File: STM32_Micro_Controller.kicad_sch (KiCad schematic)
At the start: 1 part, among them U1 STM32F103C8T6

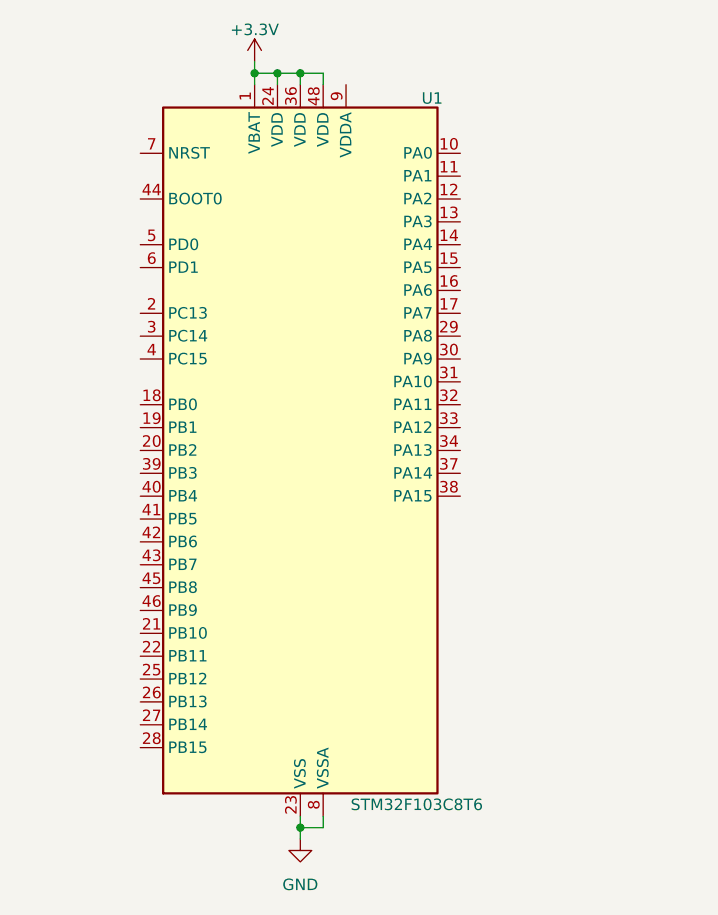
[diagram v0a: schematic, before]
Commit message: Add files via upload
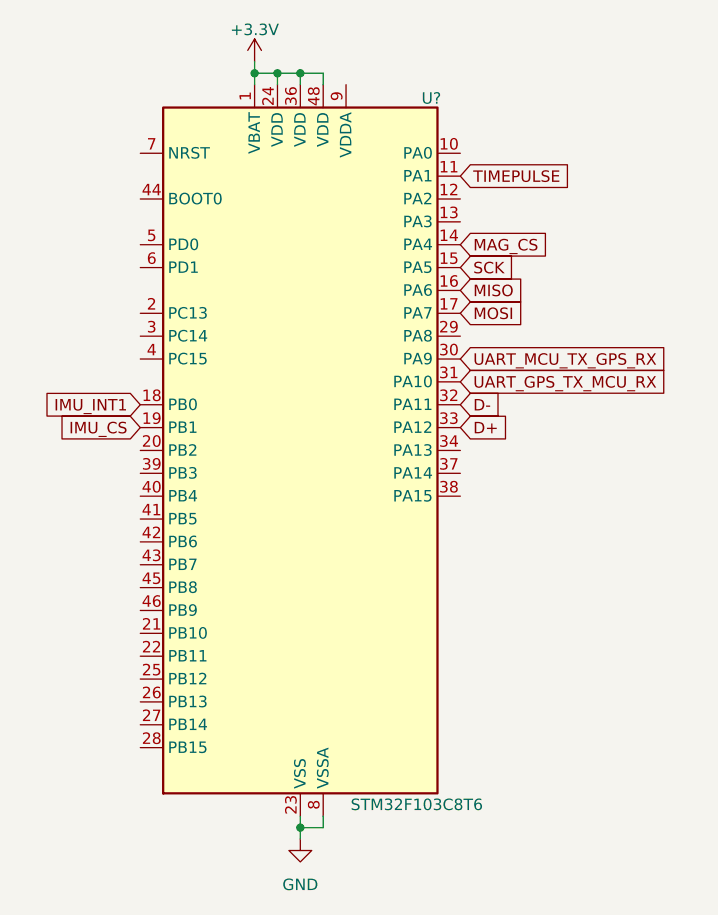
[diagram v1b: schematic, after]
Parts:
- renumbered U1 to U?
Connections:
- net TIMEPULSE: now reaches U?.11 (PA1)
- net MAG_CS: now reaches U?.14 (PA4)
- net SCK: now reaches U?.15 (PA5)
- net MISO: now reaches U?.16 (PA6)
- net MOSI: now reaches U?.17 (PA7)
- net IMU_INT1: now reaches U?.18 (PB0)
- net IMU_CS: now reaches U?.19 (PB1)
- net UART_MCU_TX_GPS_RX: now reaches U?.30 (PA9)
- net UART_GPS_TX_MCU_RX: now reaches U?.31 (PA10)
- net D-: now reaches U?.32 (PA11)
- net D+: now reaches U?.33 (PA12)

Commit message: Add files via upload
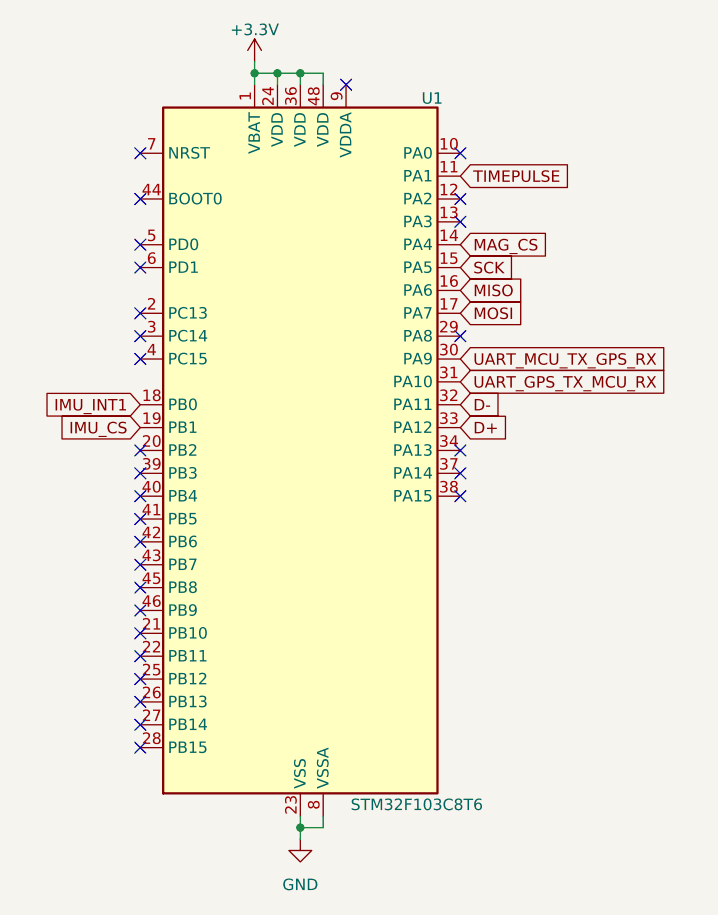
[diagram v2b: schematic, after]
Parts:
- gave numbers to parts that had none: 1
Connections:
- no-connect marks 0 -> 29
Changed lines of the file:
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@@
 		(color 0 0 0 0)
+	)
+	(no_connect
+		(at 113.03 77.47)
+	)
+	(no_connect
+		(at 113.03 102.87)
+	)
+	(no_connect
+		(at 113.03 80.01)
+	)
+	(no_connect
+		(at 113.03 64.77)
+	)
+	(no_connect
+		(at 113.03 107.95)
+	)
+	(no_connect
+		(at 135.89 52.07)
+	)
+	(no_connect
+		(at 113.03 123.19)
+	)
+	(no_connect
+		(at 113.03 115.57)
+	)
+	(no_connect
+		(at 148.59 80.01)
+	)
+	(no_connect
+		(at 113.03 113.03)
+	)
+	(no_connect
+		(at 113.03 105.41)
+	)
+	(no_connect
+		(at 113.03 125.73)
+	)
+	(no_connect
+		(at 113.03 82.55)
+	)
+	(no_connect
+		(at 113.03 120.65)
+	)
+	(no_connect
+		(at 148.59 95.25)
+	)
+	(no_connect
+		(at 148.59 97.79)
+	)
+	(no_connect
+		(at 113.03 59.69)
+	)
+	(no_connect
+		(at 148.59 64.77)
+	)
+	(no_connect
+		(at 113.03 118.11)
+	)
+	(no_connect
+		(at 148.59 92.71)
+	)
+	(no_connect
+		(at 113.03 95.25)
+	)
+	(no_connect
+		(at 113.03 97.79)
+	)
+	(no_connect
+		(at 113.03 100.33)
+	)
+	(no_connect
+		(at 113.03 72.39)
+	)
+	(no_connect
+		(at 113.03 92.71)
+	)
+	(no_connect
+		(at 113.03 110.49)
+	)
+	(no_connect
+		(at 148.59 59.69)
+	)
+	(no_connect
+		(at 148.59 67.31)
+	)
+	(no_connect
+		(at 113.03 69.85)
 	)
 	(wire
@@
 		(on_board yes)
 		(dnp no)
-		(property "Reference" "U?"
+		(property "Reference" "U1"
 			(at 144.272 53.594 0)
 			(effects
@@
 		(dnp no)
 		(fields_autoplaced yes)
-		(property "Reference" "#PWR?"
+		(property "Reference" "#PWR02"
 			(at 130.81 142.24 0)
 			(effects
@@
 			(project "flight-controller-basic"
 				(path "/e04fbe87-dc7c-407c-abef-b71ed1bbe06a/9ed827cc-d6ed-4e01-b191-8b39b0ab77a8"
-					(reference "#PWR01")
+					(reference "#PWR02")
 					(unit 1)
 				)
@@
 		(on_board yes)
 		(dnp no)
-		(property "Reference" "#PWR?"
+		(property "Reference" "#PWR01"
 			(at 125.73 53.34 0)
 			(effects
@@
 			(project "flight-controller-basic"
 				(path "/e04fbe87-dc7c-407c-abef-b71ed1bbe06a/9ed827cc-d6ed-4e01-b191-8b39b0ab77a8"
-					(reference "#PWR02")
+					(reference "#PWR01")
 					(unit 1)
 				)
